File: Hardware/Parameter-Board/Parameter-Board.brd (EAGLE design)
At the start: 100 x 80 mm, 22 parts

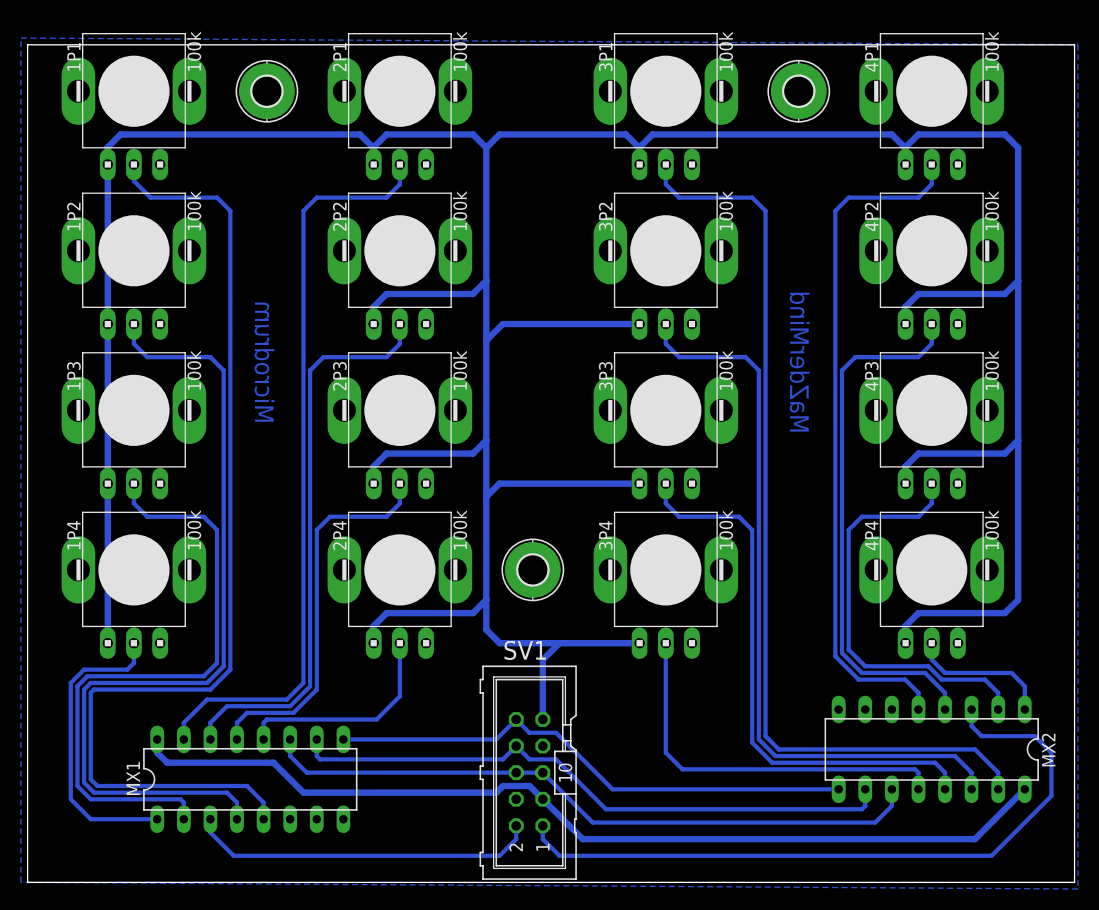
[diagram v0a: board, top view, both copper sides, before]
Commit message: Endgültiges Boardlayout
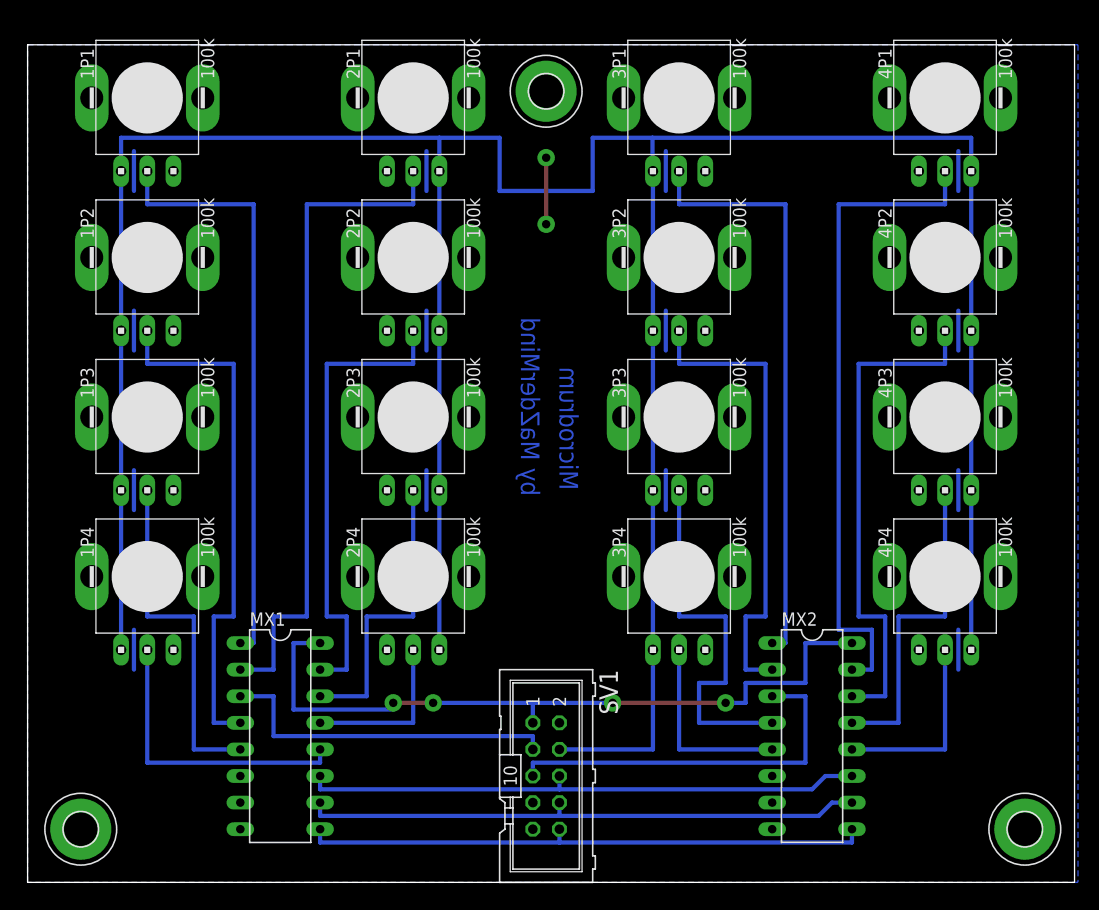
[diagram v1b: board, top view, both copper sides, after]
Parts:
- H1, H2, H3: value MOUNT-PAD-ROUND2.8 -> MOUNT-PAD-ROUND3.2; device holes:2,8-PAD -> holes:3,2-PAD
- moved H2 101.0 mm to (95.2, 5.08)
- moved H1 49.8 mm to (5.08, 5.08)
- moved H3 24.1 mm to (49.5, 75.6)
- moved MX2 11.5 mm to (74.9, 14.0), turned to 270 degrees
- moved MX1 5.02 mm to (24.1, 14.0), turned to 270 degrees
- moved SV1 1.62 mm to (49.5, 10.2), turned to 270 degrees
- moved 1P2 1.42 mm to (11.4, 59.7)
- moved 1P3 1.42 mm to (11.4, 44.5)
- moved 1P4 1.42 mm to (11.4, 29.2)
- moved 2P2 1.42 mm to (36.8, 59.7)
- moved 3P2 1.42 mm to (62.2, 59.7)
- moved 4P2 1.42 mm to (87.6, 59.7)
- moved 2P3 1.42 mm to (36.8, 44.5)
- moved 2P4 1.42 mm to (36.8, 29.2)
- moved 3P3 1.42 mm to (62.2, 44.5)
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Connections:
- net 1P2 renamed 7MX1
- removed net 1P1: 1P1.C, MX1.5
- removed net 1P3: 1P3.C, MX1.2
- removed net 1P4: 1P4.C, MX1.1
- removed net 2P1: 2P1.C, MX1.15
- removed net 2P2: 2P2.C, MX1.14
- removed net 2P3: 2P3.C, MX1.13
- removed net 2P4: 2P4.C, MX1.12
- removed net 3P1: 3P1.C, MX2.15
- removed net 3P2: 3P2.C, MX2.14
- removed net 3P3: 3P3.C, MX2.13
- removed net 3P4: 3P4.C, MX2.12
- removed net 4P1: 4P1.C, MX2.5
- removed net 4P2: 4P2.C, MX2.4
- removed net 4P3: 4P3.C, MX2.2
- removed net 4P4: 4P4.C, MX2.1
- new net 0MX1: 2P4.C, MX1.13
- new net 0MX2: 4P3.C, MX2.13
- new net 1MX1: 2P3.C, MX1.14
- new net 1MX2: 4P2.C, MX2.14
- new net 2MX1: 2P2.C, MX1.15
- new net 2MX2: 4P1.C, MX2.15
- new net 3MX1: 1P4.C, MX1.12
- new net 3MX2: 4P4.C, MX2.12
- new net 4MX1: 1P1.C, MX1.1
- new net 4MX2: 3P1.C, MX2.1
- new net 5MX1: 1P3.C, MX1.5
- new net 5MX2: 3P4.C, MX2.5
- new net 6MX1: 2P1.C, MX1.2
- new net 6MX2: 3P2.C, MX2.2
- new net 7MX2: 3P3.C, MX2.4
- net A: no longer SV1.5
- net AGND: now also 2P1.B, 2P2.B, 2P3.B, 2P4.B, 4P1.B, 4P2.B, 4P3.B, 4P4.B, SV1.4; no longer 2P1.A, 2P2.A, 2P3.A, 2P4.A, 4P1.A, 4P2.A, 4P3.A, 4P4.A, SV1.9
- net GND: now also 2P1.A, 2P2.A, 2P3.A, 2P4.A, 4P1.A, 4P2.A, 4P3.A, 4P4.A, SV1.2; no longer 2P1.B, 2P2.B, 2P3.B, 2P4.B, 4P1.B, 4P2.B, 4P3.B, 4P4.B, SV1.4
- net VCC: now also SV1.1; no longer SV1.3
- net X1: now also SV1.3; no longer SV1.2
- net X2: now also SV1.5; no longer SV1.1
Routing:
- net 1P1: track 97.3 -> 0.00 mm
- net 3P1: track 87.9 -> 0.00 mm
- net 2P1: track 71.8 -> 0.00 mm
- net 3P2: track 70.3 -> 0.00 mm
- net 4P1: track 65.7 -> 0.00 mm
- net AGND: track 369.6 -> 305.5 mm
- net 6MX1: track 0.00 -> 64.1 mm
- net 2MX2: track 0.00 -> 62.9 mm
- net 1P3: track 59.8 -> 0.00 mm
- net GND: track 0.00 -> 59.7 mm, vias 0 -> 2
- net 4MX2: track 0.00 -> 56.5 mm
- net 4MX1: track 0.00 -> 56.5 mm
- net 2P2: track 54.2 -> 0.00 mm
- net 3P3: track 52.7 -> 0.00 mm
- net 4P2: track 51.5 -> 0.00 mm
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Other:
- board text added: "by MaZderMind"
- board text removed: "MaZderMind"
